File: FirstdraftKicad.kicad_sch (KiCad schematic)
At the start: 27 parts, among them J1 Conn_Coaxial, J2 Conn_Coaxial, U1 Opamp_Quad

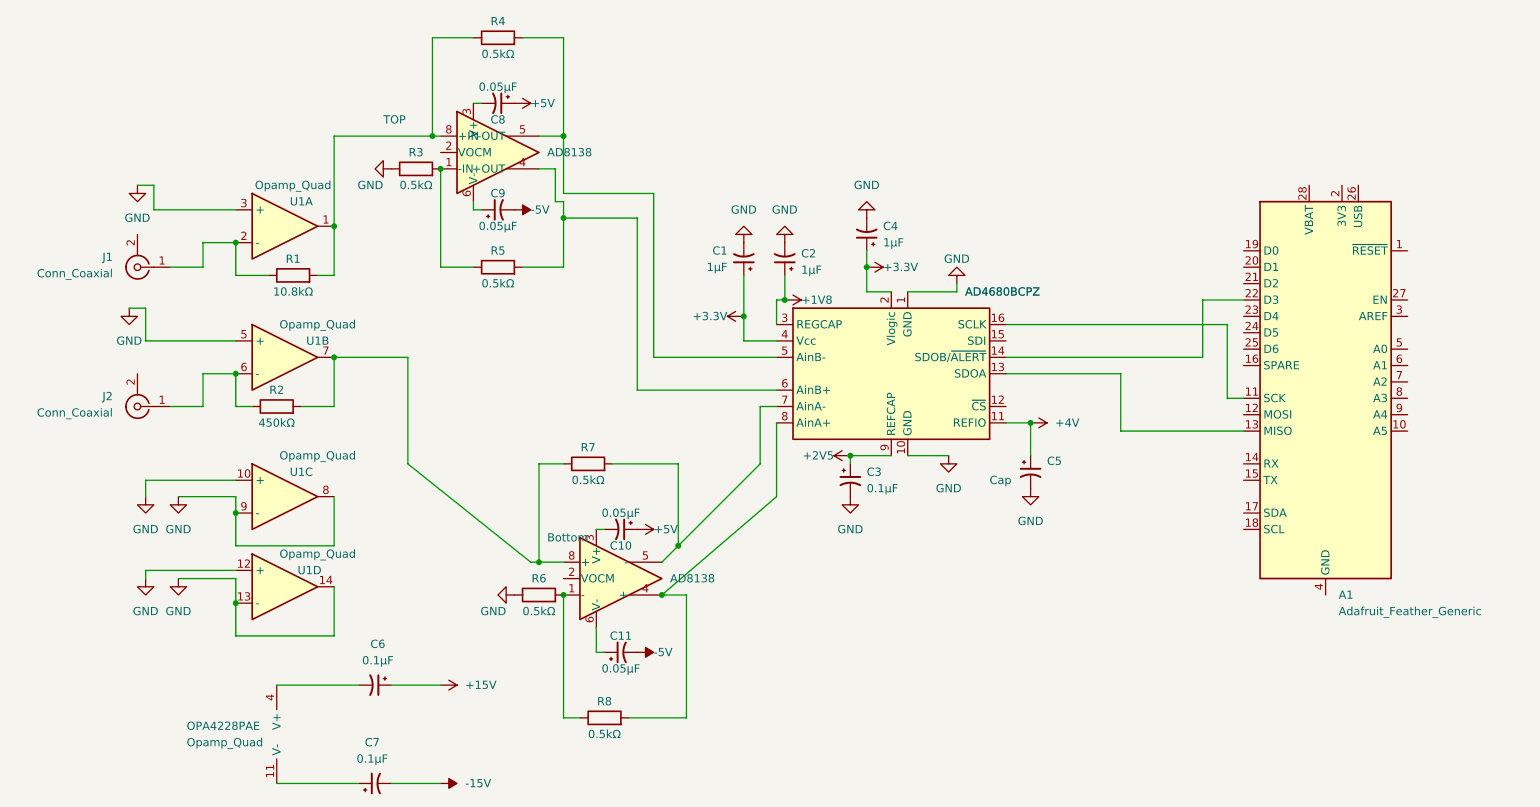
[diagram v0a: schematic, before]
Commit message: Updated kicad files
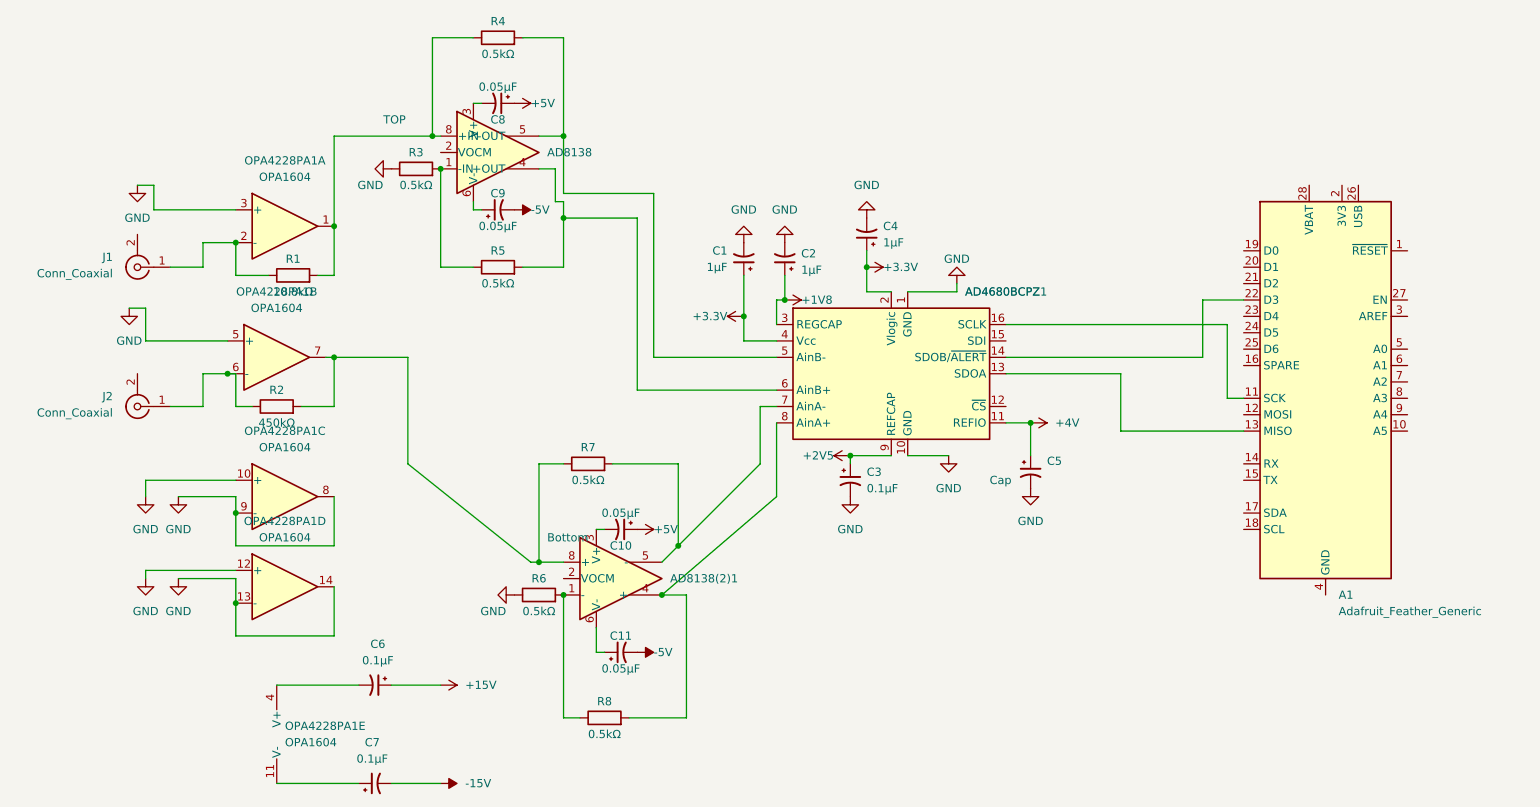
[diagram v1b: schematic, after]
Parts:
- removed OPA4228PA, U1: Opamp_Quad, Package_DIP:DIP-14_W7.62mm, symbol Device:Opamp_Quad
- added OPA4228PA1: OPA1604, Package_DIP:DIP-14_W7.62mm, symbol Amplifier_Operational:OPA1604
- J1, J2: footprint Connector_Coaxial:BNC_PanelMountable_Vertical -> Connector_Coaxial:MMCX_Molex_73415-1471_Vertical
- renumbered AD4680BCPZ to AD4680BCPZ1, AD8138 to AD8138(2)1
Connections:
- net GND: now also OPA4228PA1.10 (+), OPA4228PA1.12 (+), OPA4228PA1.13 (-), OPA4228PA1.14, OPA4228PA1.3 (+), OPA4228PA1.5 (+), OPA4228PA1.8, OPA4228PA1.9 (-)
- net at J2.1 (In), R2.1: now also OPA4228PA1.6 (-)
- net at AD8138(2)1.8 (+), R2.2, R7.1: now also OPA4228PA1.7
- net at J1.1 (In), R1.1: now also OPA4228PA1.2 (-)
- net at C6.2: now also OPA4228PA1.4 (V+)
- net at C7.1: now also OPA4228PA1.11 (V-)
- net at AD8138.8 (+IN), R1.2, R4.1: now also OPA4228PA1.1
